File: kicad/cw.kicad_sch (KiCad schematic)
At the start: 110 parts, among them J1 AUDIO, J2 KEY, Q1 NPN, Q10 NPN, Q11 NPN, Q2 NMOS, Q3 NPN, Q4 NPN, Q6 NPN, Q7 NPN, Q8 NPN, Q9 NPN, SW1 TX/RX, SW2 TX/RX, SW3 FREQ_SELECT, U1 Si5351A-B-GT, U3 PCF8574TS, U4 RC1602A, Y1 4M, Y2 4M, Y3 4M, Y4 4M, Y5 4M, Y6 4M, Y7 4M, Y8 4M

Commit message: Update cw.kicad_sch
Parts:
- removed C35: 100n, symbol Device:C
- added Y10, Y11, Y12, Y13, Y14, Y15, Y9: 4M, symbol Device:Crystal
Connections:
- net at Q3.2 (B), R3.1, Y5.1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: now also Y13.1, Y14.1, Y15.1
- net at C1.1, C12.1, C16.1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: now also Y13.2, Y14.2, Y15.2
- net at Q1.3 (E), R22.1: now also L19.1
- net at J2.T, Y1.1, Y2.1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: now also Y10.1, Y11.1, Y12.1, Y9.1
- net at C9.1, Y1.2, Y2.2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: now also Y10.2, Y11.2, Y12.2, Y9.2; no longer C29.1
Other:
- moved on the sheet: C10, C11, C18, C19, C2, C20, C22, C3, C4, C6, C9, D2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

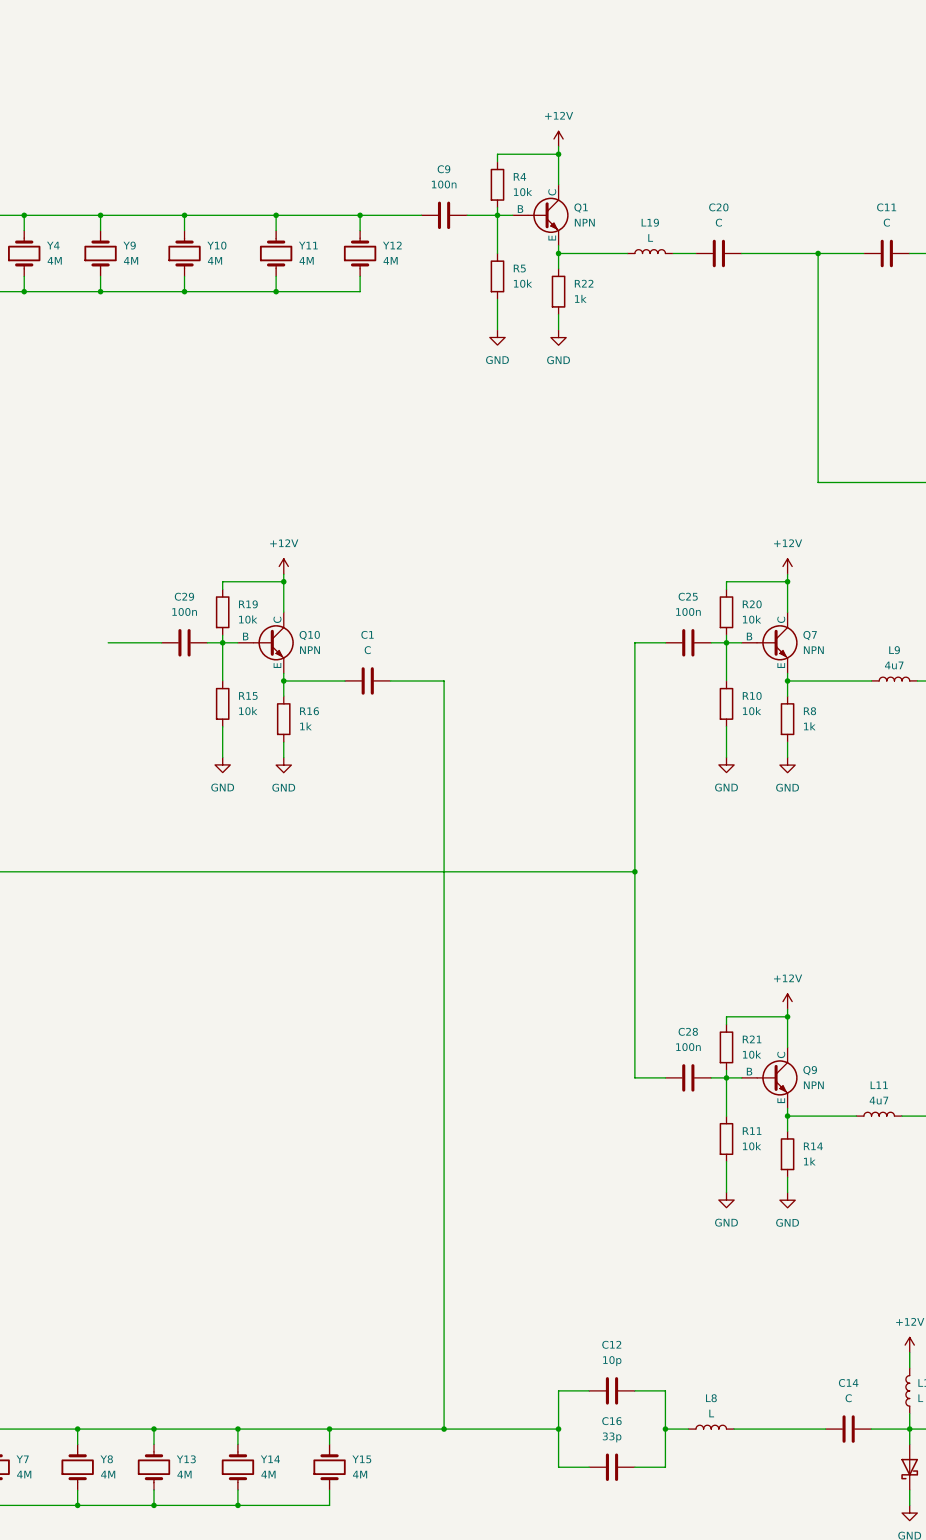
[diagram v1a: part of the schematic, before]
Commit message: Update cw.kicad_sch
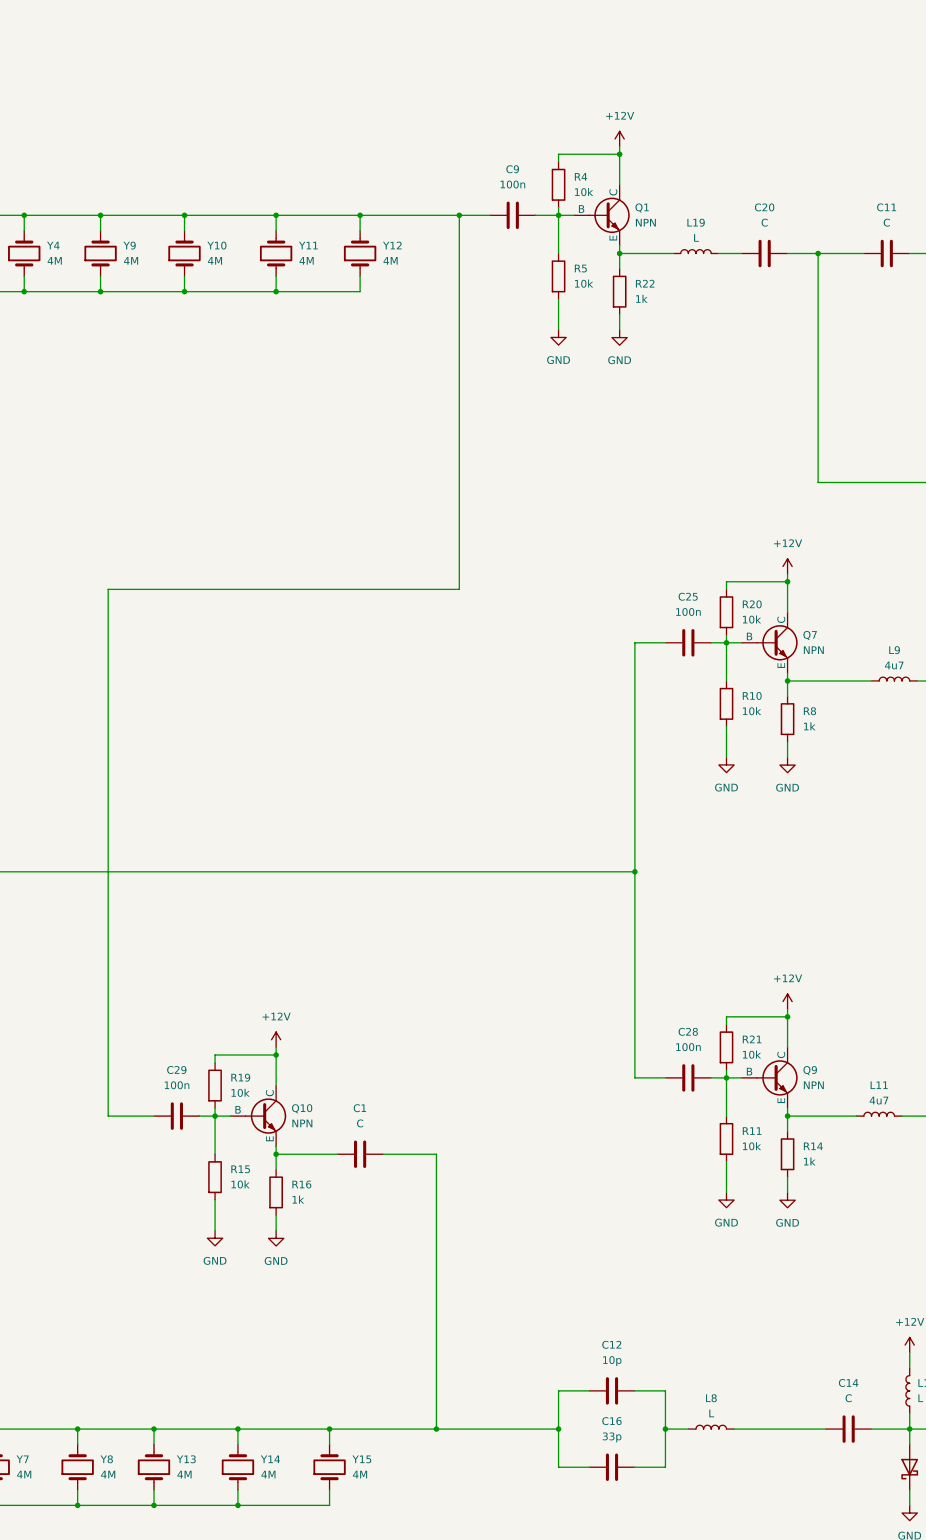
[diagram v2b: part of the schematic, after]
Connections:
- net at C9.1, Y1.2, Y10.2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: now also C29.1
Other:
- moved on the sheet: C1, C20, C29, C9, L19, Q1, Q10, R15, R16, R19, R22, R4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

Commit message: Update cw.kicad_sch
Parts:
- added Y16: 4M, symbol Device:Crystal
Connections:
- net at Q3.2 (B), R3.1, Y13.1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: now also Y16.1
- net at C1.1, C12.1, C16.1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: now also Y16.2
- net at Y1.1, Y10.1, Y11.1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: now also J2.S; no longer J2.T
- net at C23.2, C41.2: now also J2.T; no longer J2.S
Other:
- moved on the sheet: AE1, C1, C10, C11, C12, C13, C14, C15, C16, C17, C18, C19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
